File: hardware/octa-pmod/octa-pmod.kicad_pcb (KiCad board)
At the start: 2 copper layers, 54.5 x 46.4 mm, 19 parts, among them J1 PMOD, J10 PMOD, J12 PWR, J14 PWR, J15 PMOD, J16 PMOD, J2 PMOD, J3 S7 Mini, J4 S7 Mini, J5 PWR, J6 PWR, J7 PMOD, J8 PMOD, J9 PMOD, M1 M3, M2 M3, M3 M3, M4 M3

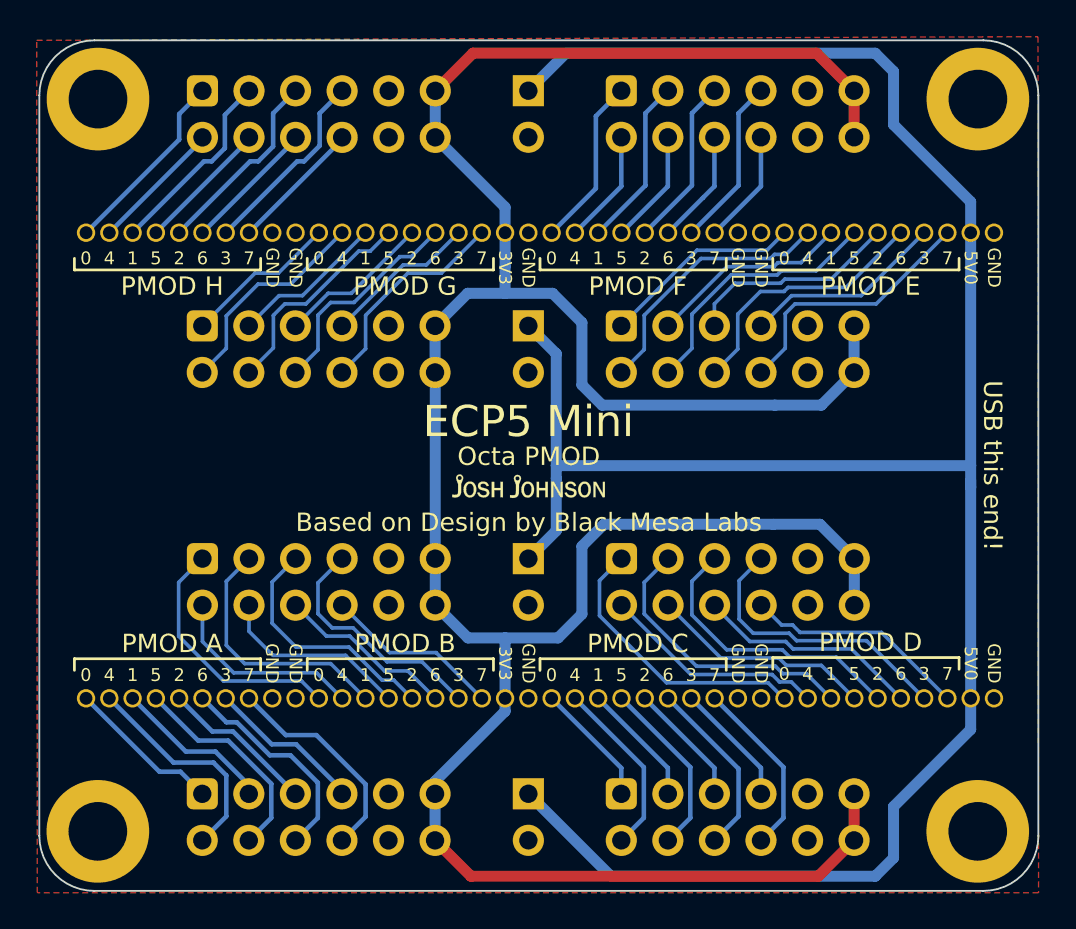
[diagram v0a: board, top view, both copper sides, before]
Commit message: clean up routing
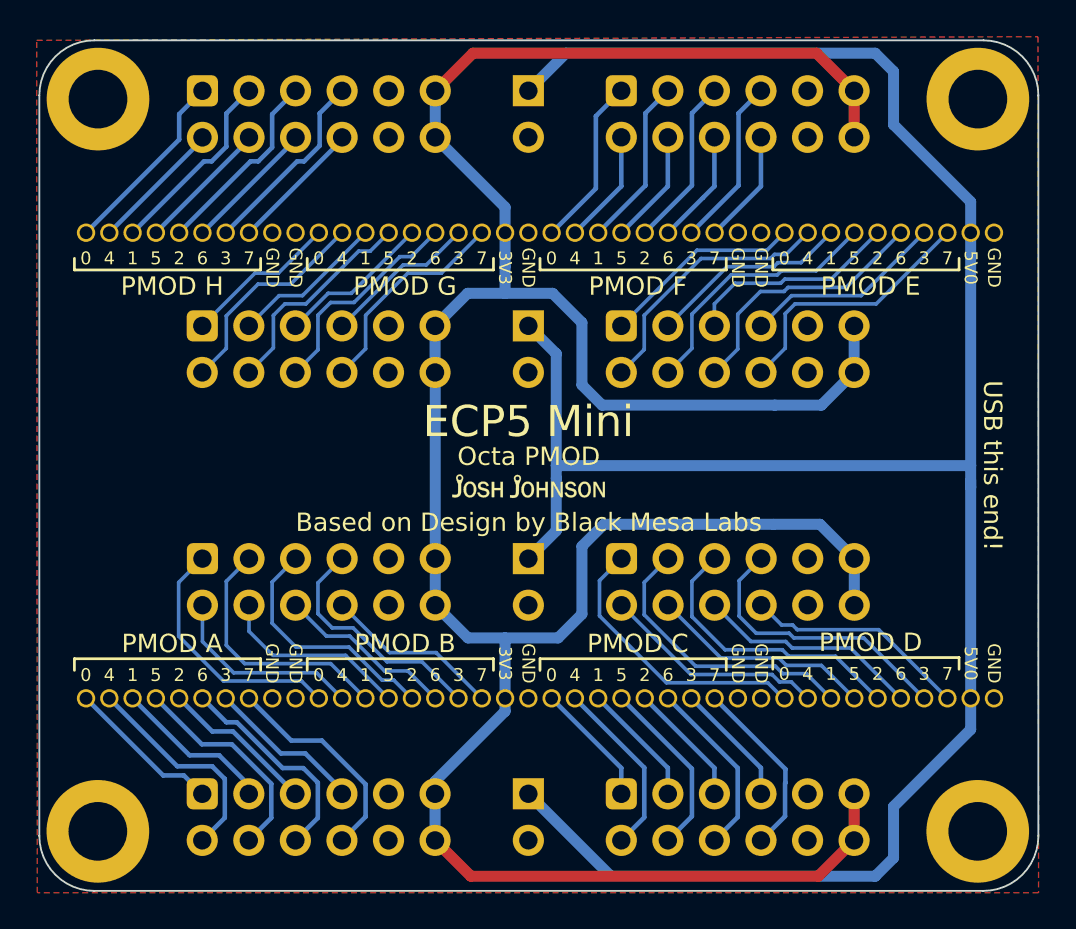
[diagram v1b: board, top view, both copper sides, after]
